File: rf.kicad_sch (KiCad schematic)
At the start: 3 parts, among them J1 ANT_A, J2 ANT_B

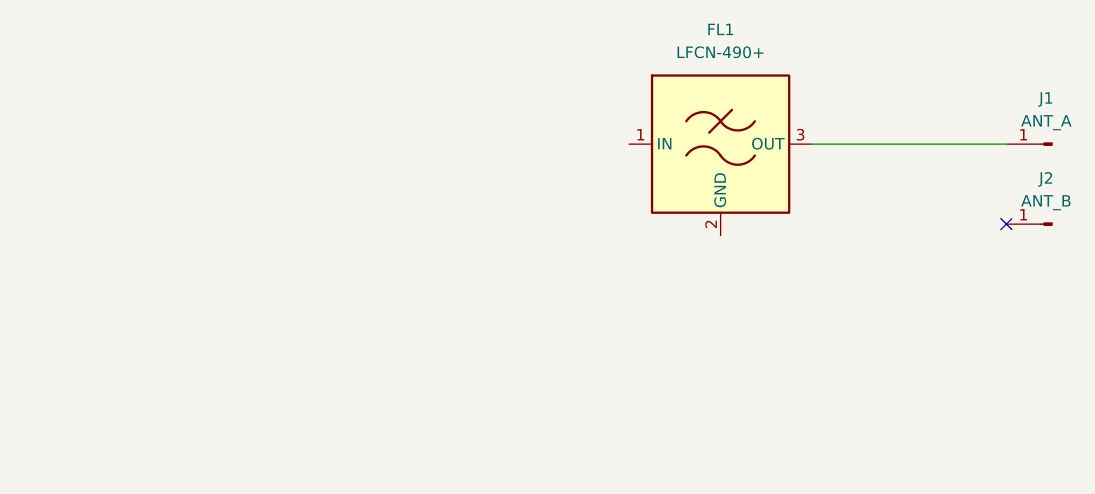
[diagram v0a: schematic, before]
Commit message: more stuff
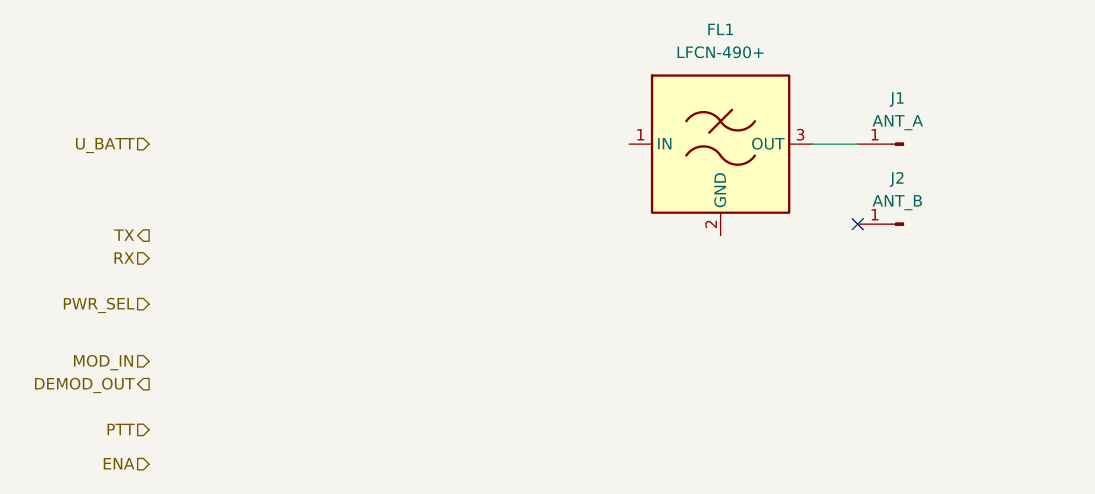
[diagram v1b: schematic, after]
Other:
- moved on the sheet: J1, J2
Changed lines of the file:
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@@
 	)
 	(no_connect
-		(at 196.85 93.98)
+		(at 180.34 93.98)
 	)
 	(wire
 		(pts
-			(xy 175.26 85.09) (xy 196.85 85.09)
+			(xy 175.26 85.09) (xy 180.34 85.09)
 		)
 		(stroke
@@
 		)
 	)
+	(hierarchical_label "TX"
+		(shape output)
+		(at 101.6 95.25 180)
+		(fields_autoplaced yes)
+		(effects
+			(font
+				(size 1.27 1.27)
+			)
+			(justify right)
+		)
+	)
+	(hierarchical_label "DEMOD_OUT"
+		(shape output)
+		(at 101.6 111.76 180)
+		(fields_autoplaced yes)
+		(effects
+			(font
+				(size 1.27 1.27)
+			)
+			(justify right)
+		)
+	)
+	(hierarchical_label "U_BATT"
+		(shape input)
+		(at 101.6 85.09 180)
+		(fields_autoplaced yes)
+		(effects
+			(font
+				(size 1.27 1.27)
+			)
+			(justify right)
+		)
+	)
+	(hierarchical_label "PWR_SEL"
+		(shape input)
+		(at 101.6 102.87 180)
+		(fields_autoplaced yes)
+		(effects
+			(font
+				(size 1.27 1.27)
+			)
+			(justify right)
+		)
+	)
+	(hierarchical_label "ENA"
+		(shape input)
+		(at 101.6 120.65 180)
+		(fields_autoplaced yes)
+		(effects
+			(font
+				(size 1.27 1.27)
+			)
+			(justify right)
+		)
+	)
+	(hierarchical_label "MOD_IN"
+		(shape input)
+		(at 101.6 109.22 180)
+		(fields_autoplaced yes)
+		(effects
+			(font
+				(size 1.27 1.27)
+			)
+			(justify right)
+		)
+	)
+	(hierarchical_label "PTT"
+		(shape input)
+		(at 101.6 116.84 180)
+		(fields_autoplaced yes)
+		(effects
+			(font
+				(size 1.27 1.27)
+			)
+			(justify right)
+		)
+	)
+	(hierarchical_label "RX"
+		(shape input)
+		(at 101.6 97.79 180)
+		(fields_autoplaced yes)
+		(effects
+			(font
+				(size 1.27 1.27)
+			)
+			(justify right)
+		)
+	)
 	(symbol
 		(lib_id "Connector:Conn_01x01_Pin")
-		(at 201.93 85.09 180)
+		(at 185.42 85.09 180)
 		(unit 1)
 		(exclude_from_sim no)
@@
 		(fields_autoplaced yes)
 		(property "Reference" "J1"
-			(at 201.295 80.01 0)
+			(at 184.785 80.01 0)
 			(effects
 				(font
@@
 		)
 		(property "Value" "ANT_A"
-			(at 201.295 82.55 0)
+			(at 184.785 82.55 0)
 			(effects
 				(font
@@
 		)
 		(property "Footprint" "TestPoint:TestPoint_Pad_D2.5mm"
-			(at 201.93 85.09 0)
+			(at 185.42 85.09 0)
 			(effects
 				(font
@@
 		)
 		(property "Datasheet" "~"
-			(at 201.93 85.09 0)
+			(at 185.42 85.09 0)
 			(effects
 				(font
@@
 		)
 		(property "Description" "Generic connector, single row, 01x01, script generated"
-			(at 201.93 85.09 0)
+			(at 185.42 85.09 0)
 			(effects
 				(font
@@
 	(symbol
 		(lib_id "Connector:Conn_01x01_Pin")
-		(at 201.93 93.98 180)
+		(at 185.42 93.98 180)
 		(unit 1)
 		(exclude_from_sim no)
@@
 		(fields_autoplaced yes)
 		(property "Reference" "J2"
-			(at 201.295 88.9 0)
+			(at 184.785 88.9 0)
 			(effects
 				(font
@@
 		)
 		(property "Value" "ANT_B"
-			(at 201.295 91.44 0)
+			(at 184.785 91.44 0)
 			(effects
 				(font
@@
 		)
 		(property "Footprint" "TestPoint:TestPoint_Pad_D2.5mm"
-			(at 201.93 93.98 0)
+			(at 185.42 93.98 0)
 			(effects
 				(font
@@
 		)
 		(property "Datasheet" "~"
-			(at 201.93 93.98 0)
+			(at 185.42 93.98 0)
 			(effects
 				(font
@@
 		)
 		(property "Description" "Generic connector, single row, 01x01, script generated"
-			(at 201.93 93.98 0)
-			(effects
-				(font
+			(at 185.42 93.98 0)
+			(effects
+				(font
